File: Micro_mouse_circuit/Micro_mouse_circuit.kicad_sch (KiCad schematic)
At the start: 26 parts, among them J1 Conn_02x16_Odd_Even, J2 Battery input, J3 USB_C_Receptacle_PowerOnly_6P, J4 Conn_01x02, SW1 SW_SP3T, U1 LM2596SX-5_0/NOPB, U2 INA219AxDCN, U3 HUSB237-AA001-DN06R, U4 TP4056_C382139, U5 TYPE-C_6P_LTH6_5, U6 SN74LVC1G3157DCKR

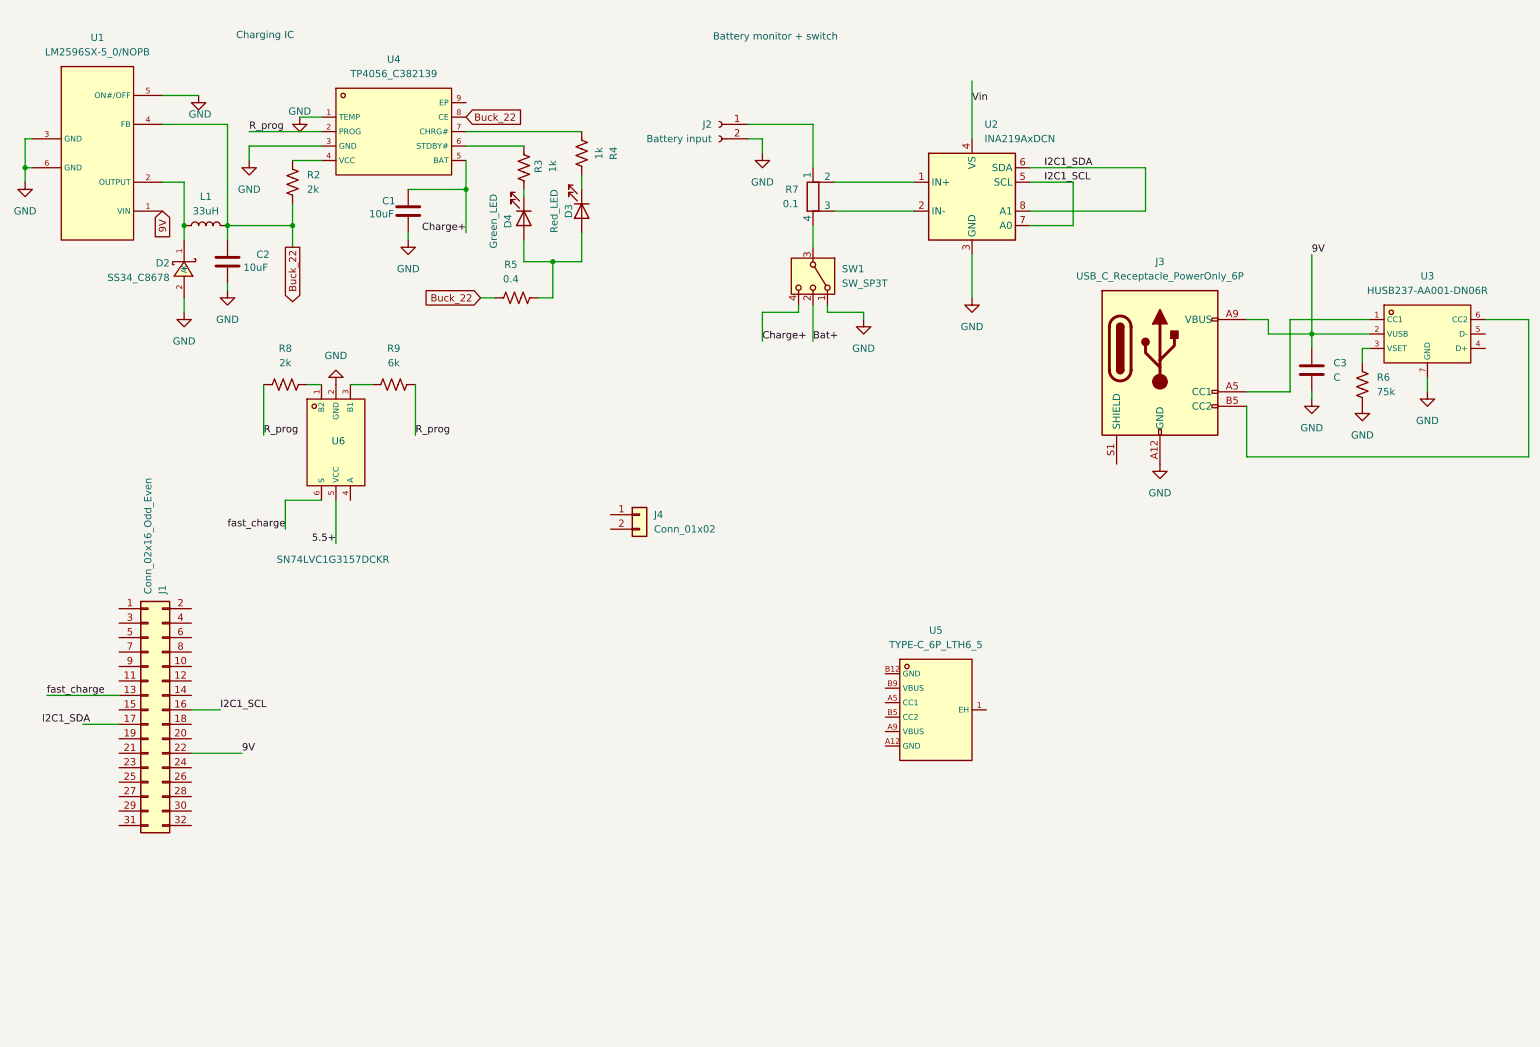
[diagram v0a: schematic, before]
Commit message: began schematic rev 3.0
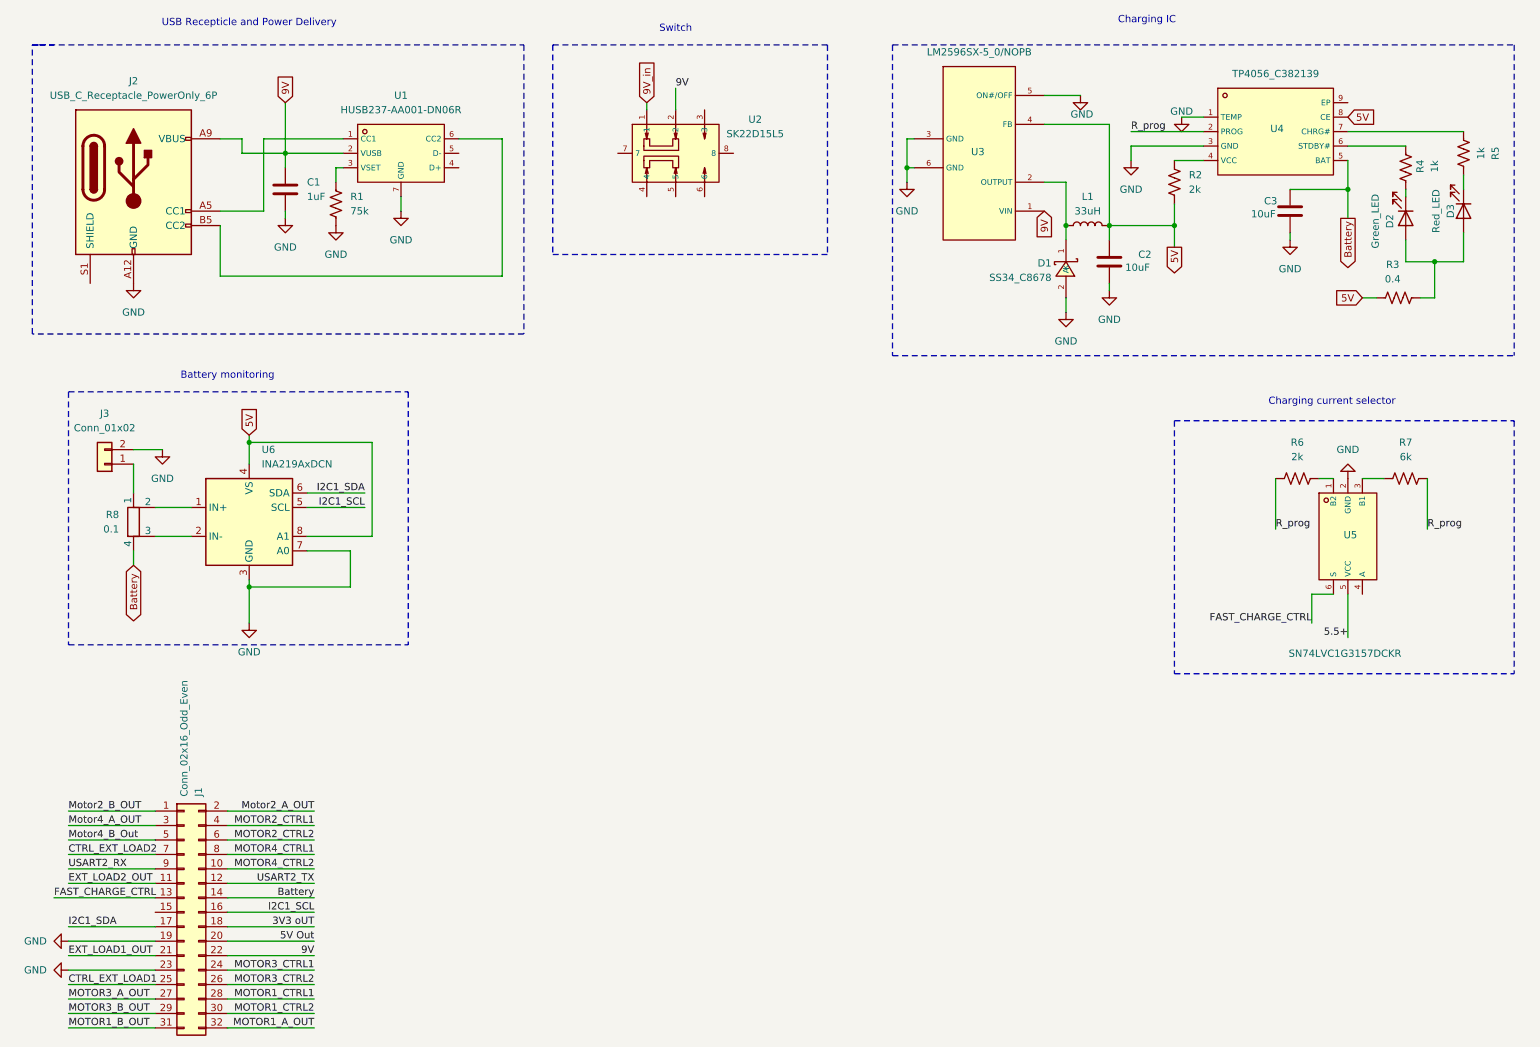
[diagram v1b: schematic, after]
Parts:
- removed D2: SS34_C8678, xxcustom_footprint:SMA_L4.3-W2.6-LS5.2-RD, symbol SS34_C8678:SS34_C8678
- removed D4: Green_LED, symbol Device:LED
- removed J2: Battery input, Connector_Wire:SolderWire-0.127sqmm_1x02_P3.7mm_D0.48mm_OD1mm, symbol Connector:Conn_01x02_Socket
- removed J3: USB_C_Receptacle_PowerOnly_6P, symbol Connector:USB_C_Receptacle_PowerOnly_6P
- removed J4: Conn_01x02, Connector_JST:JST_PH_S2B-PH-K_1x02_P2.00mm_Horizontal, symbol Connector_Generic:Conn_01x02
- removed R7: 0.1, symbol Device:R_Shunt
- removed R8: 2k, xxcustom_footprint:R0402, symbol Device:R_US
- removed R9: 6k, xxcustom_footprint:R0402, symbol Device:R_US
- removed SW1: SW_SP3T, symbol Switch:SW_SP3T
- removed U1: LM2596SX-5_0/NOPB, xxcustom_footprint:TO-263-5_L10.2-W8.9-P1.70-TL, symbol LM2596SX-5_0/NOPB:LM2596SX-5_0/NOPB
- removed U2: INA219AxDCN, Package_TO_SOT_SMD:SOT-23-8, symbol Sensor_Energy:INA219AxDCN
- removed U3: HUSB237-AA001-DN06R, xxcustom_footprint:TDFN-6_L2.0-W2.0-P0.65-TL-EP, symbol HUSB237-AA001-DN06R:HUSB237-AA001-DN06R
- removed U5: TYPE-C_6P_LTH6_5, xxcustom_footprint:USB-TYPE-C-SMD_TYPE-C-6P-LTH6.5, symbol TYPE-C_6P_LTH6_5:TYPE-C_6P_LTH6_5
- removed U6: SN74LVC1G3157DCKR, xxcustom_footprint:SC-70-6_L2.2-W1.3-P0.65-LS2.1-BR, symbol SN74LVC1G3157DCKR:SN74LVC1G3157DCKR
- added D1: SS34_C8678, xxcustom_footprint:SMA_L4.3-W2.6-LS5.2-RD, symbol SS34_C8678:SS34_C8678
- added D2: Green_LED, symbol Device:LED
- added J2: USB_C_Receptacle_PowerOnly_6P, symbol Connector:USB_C_Receptacle_PowerOnly_6P
- added J3: Conn_01x02, Connector_JST:JST_PH_S2B-PH-K_1x02_P2.00mm_Horizontal, symbol Connector_Generic:Conn_01x02
- added R1: 75k, symbol Device:R_US
- added R7: 6k, xxcustom_footprint:R0402, symbol Device:R_US
- added R8: 0.1, symbol Device:R_Shunt
- added U1: HUSB237-AA001-DN06R, xxcustom_footprint:TDFN-6_L2.0-W2.0-P0.65-TL-EP, symbol HUSB237-AA001-DN06R:HUSB237-AA001-DN06R
- added U2: SK22D15L5, xxcustom_footprint:SW-TH_XKB_SK22D15L7, symbol SK22D15L5:SK22D15L5
- added U3: LM2596SX-5_0/NOPB, xxcustom_footprint:TO-263-5_L10.2-W8.9-P1.70-TL, symbol LM2596SX-5_0/NOPB:LM2596SX-5_0/NOPB
- added U5: SN74LVC1G3157DCKR, xxcustom_footprint:SC-70-6_L2.2-W1.3-P0.65-LS2.1-BR, symbol SN74LVC1G3157DCKR:SN74LVC1G3157DCKR
- added U6: INA219AxDCN, Package_TO_SOT_SMD:SOT-23-8, symbol Sensor_Energy:INA219AxDCN
- C1: value 10uF -> 1uF
- C3: value C -> 10uF
- R3: value 1k -> 0.4; footprint xxcustom_footprint:R0402 -> (none)
- R5: value 0.4 -> 1k; footprint (none) -> xxcustom_footprint:R0402
- R6: value 75k -> 2k; footprint (none) -> xxcustom_footprint:R0402
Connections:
- net 5.5+: now also U5.5 (VCC)
- net 9V: now also C1.1, J2.A9 (VBUS), J2.B9 (VBUS), U1.2 (VUSB), U2.2, U3.1 (VIN); no longer C3.1
- net GND: now also J1.19 (Pin_19), J1.23 (Pin_23), D1.2 (A), J2.A12 (GND), J2.B12 (GND), J3.2 (Pin_2), R1.2, U1.7 (GND), U3.3 (GND), U3.5 (ON#/OFF), U3.6 (GND), U5.2 (GND), U6.3 (GND), U6.7 (A0); no longer R6.2
- net I2C1_SCL: now also U6.5 (SCL)
- net I2C1_SDA: now also U6.6 (SDA)
- net R_prog: now also R6.1, R7.1
- net at R4.1: now also U4.6 (STDBY#); no longer D3.1 (K)
- net at R4.2: now also D2.1 (K); no longer U4.7 (CHRG#)
- net at L1.1: now also D1.1 (K), U3.2 (OUTPUT)
- net at D3.2 (A): now also R3.2, D2.2 (A); no longer R5.2
- net 5V: now reaches R3.1
- net 5V: now also C2.1, L1.2, R2.1, U4.8 (CE), U3.4 (FB), U6.4 (VS), U6.8 (A1); no longer U4.6 (STDBY#)
- net Motor2_B_OUT: now reaches J1.1 (Pin_1)
- net MOTOR4_CTRL2: now reaches J1.10 (Pin_10)
- net EXT_LOAD2_OUT: now reaches J1.11 (Pin_11)
- net USART2_TX: now reaches J1.12 (Pin_12)
- net Battery: now reaches J1.14 (Pin_14)
- net Battery: now also C3.1, U4.5 (BAT), R8.4
- net 3V3 oUT: now reaches J1.18 (Pin_18)
- net Motor2_A_OUT: now reaches J1.2 (Pin_2)
- net 5V Out: now reaches J1.20 (Pin_20)
- net EXT_LOAD1_OUT: now reaches J1.21 (Pin_21)
- net MOTOR3_CTRL1: now reaches J1.24 (Pin_24)
- net CTRL_EXT_LOAD1: now reaches J1.25 (Pin_25)
- net MOTOR3_CTRL2: now reaches J1.26 (Pin_26)
- net MOTOR3_A_OUT: now reaches J1.27 (Pin_27)
- net MOTOR1_CTRL1: now reaches J1.28 (Pin_28)
- net MOTOR3_B_OUT: now reaches J1.29 (Pin_29)
- net Motor4_A_OUT: now reaches J1.3 (Pin_3)
- net MOTOR1_CTRL2: now reaches J1.30 (Pin_30)
- net MOTOR1_B_OUT: now reaches J1.31 (Pin_31)
- net MOTOR1_A_OUT: now reaches J1.32 (Pin_32)
- net MOTOR2_CTRL1: now reaches J1.4 (Pin_4)
- net Motor4_B_Out: now reaches J1.5 (Pin_5)
- net MOTOR2_CTRL2: now reaches J1.6 (Pin_6)
- net CTRL_EXT_LOAD2: now reaches J1.7 (Pin_7)
- net MOTOR4_CTRL1: now reaches J1.8 (Pin_8)
- net USART2_RX: now reaches J1.9 (Pin_9)
- removed net Buck_22: C2.1, L1.2, R2.1, R5.1, U4.8 (CE)
- removed net Charge+: C1.1, U4.5 (BAT)
- net fast_charge renamed FAST_CHARGE_CTRL
- net FAST_CHARGE_CTRL: now also U5.6 (S)
- new net: J3.1 (Pin_1), R8.1
- new net: R7.2, U5.3 (B1)
- new net: R6.2, U5.1 (B2)
- new net: R1.1, U1.3 (VSET)
- new net: J2.A5 (CC1), U1.1 (CC1)
- new net: J2.B5 (CC2), U1.6 (CC2)
- new net: R8.2, U6.1 (IN+)
- new net: R8.3, U6.2 (IN-)
- new net: R5.2, U4.7 (CHRG#)
- new net: D3.1 (K), R5.1
- new net 9V_in: U2.1
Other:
- note added: "Battery monitoring"
- note added: "Charging current selector"
- note added: "Switch"
- note added: "USB Recepticle and Power Delivery"
- note removed: "Battery monitor + switch"
- company: (none) -> University of Cape Town
- title: EEE3088_Micro_Mouse_Power_Sub_system -> EEE3088_Micro_Mouse_PCB
